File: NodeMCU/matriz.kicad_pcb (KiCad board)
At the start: 2 copper layers, 68 x 68 mm, 26 parts, among them J1 Conn_01x05, J2 Conn_01x02, Q1 Q_NPN_CBE, Q2 Q_NPN_CBE, Q3 Q_NPN_CBE, SW1 SW_Push_Open, SW2 SW_Push, U3 NodeMCU1.0(ESP-12E)

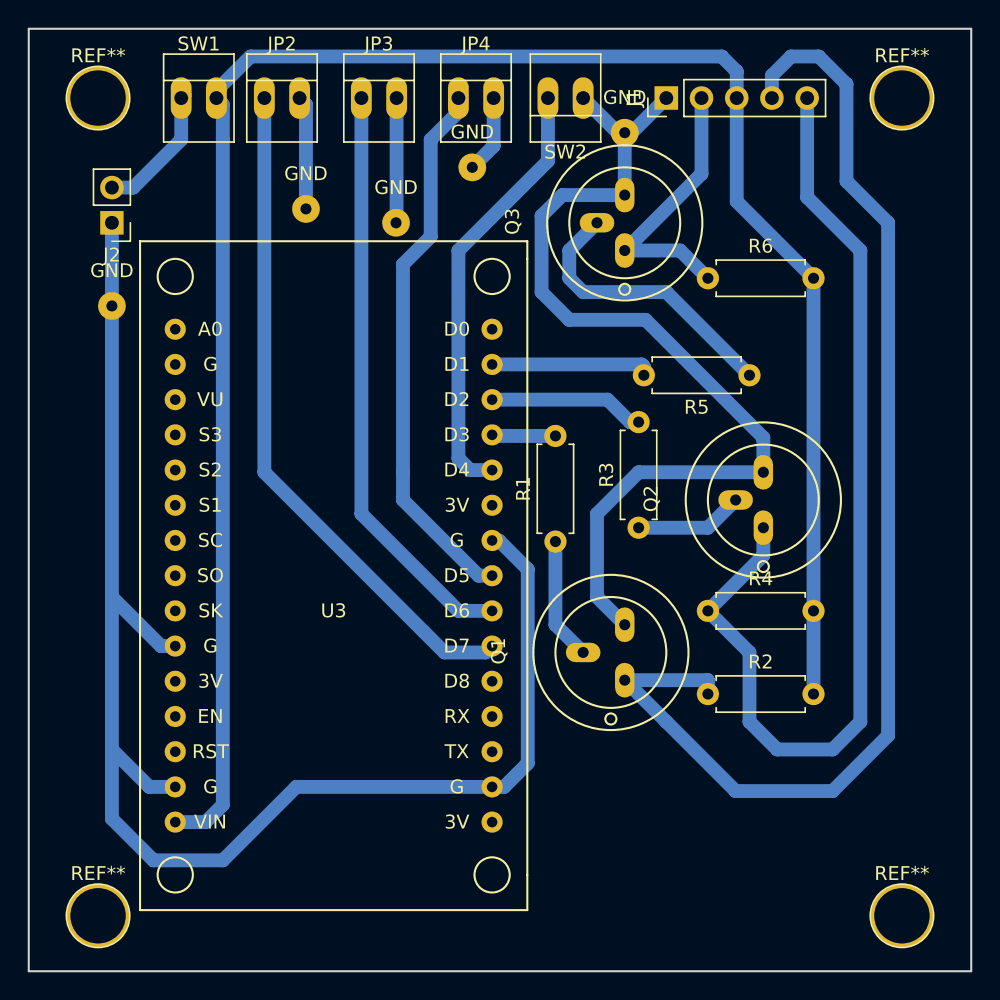
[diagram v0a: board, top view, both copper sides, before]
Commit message: Pads adecuados
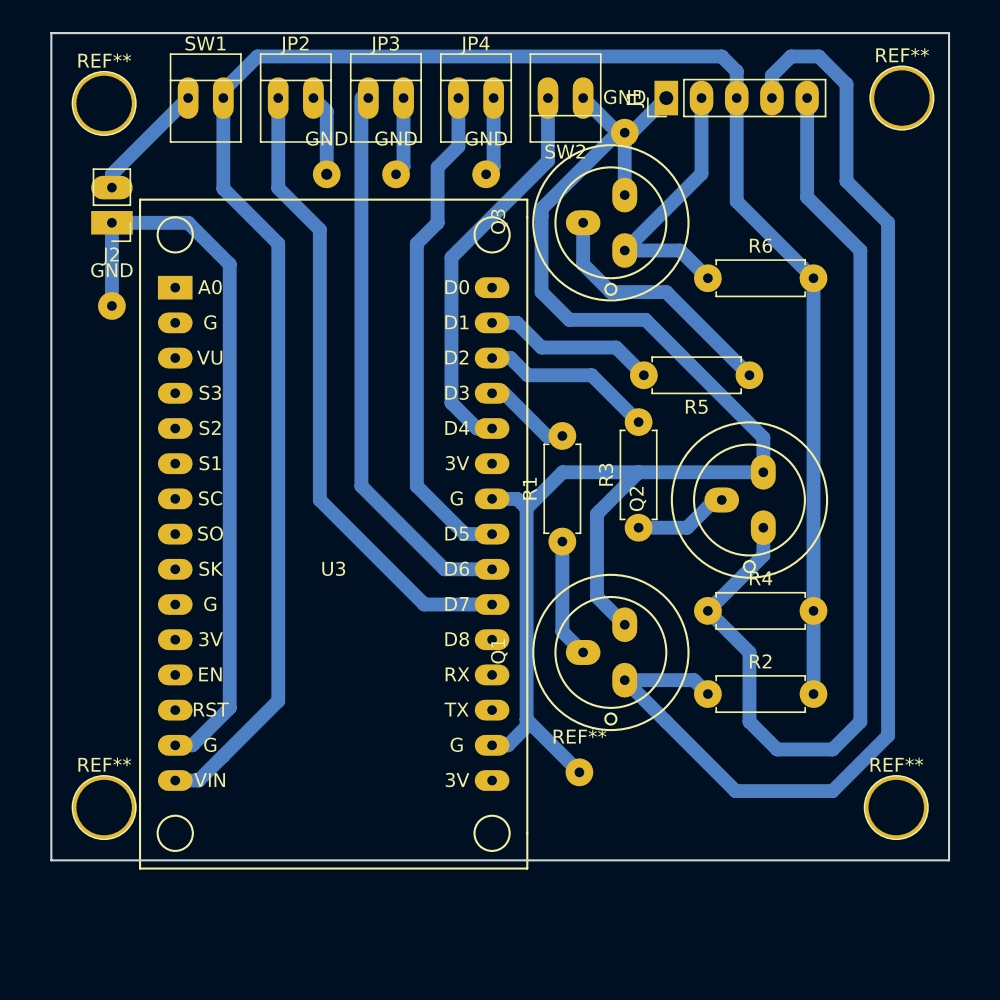
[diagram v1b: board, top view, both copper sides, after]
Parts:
- added REF**: SolderWirePad_single_0-8mmDrill, Wire_Pads:SolderWirePad_single_0-8mmDrill, F.Cu at (125.7, 120.7)
- R1, R3, R5: value 500Ohm -> 10KOhm
- R2, R6: value 1000KOhm -> 10KOhm
- R4: value 1000Ohm -> 10KOhm
- moved REF** 7.82 mm to (91.4, 123.2)
- moved REF** 7.82 mm to (148.6, 123.2)
- moved GND 3.50 mm to (112.5, 77.5)
- moved U3 3.00 mm to (108.0, 106.0)
- moved GND 2.92 mm to (107.5, 77.5)
- moved GND 1.12 mm to (119.0, 77.5)
- moved JP2 1.00 mm to (104.0, 72.0)
- moved Q2 1.00 mm to (138.0, 101.0)
- moved Q3 1.00 mm to (128.0, 81.0)
- moved REF** 0.59 mm to (91.4, 72.4)
- moved JP3 0.50 mm to (110.5, 72.0)
- moved R1 0.50 mm to (124.5, 104.0)
- moved SW1 0.50 mm to (97.5, 72.0)
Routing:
- net /GND: track 199.2 -> 178.4 mm
- net Net-(JP4-Pad1): track 39.3 -> 36.1 mm
- net Net-(JP2-Pad1): track 49.0 -> 45.8 mm
- net Net-(SW2-Pad2): track 31.5 -> 28.6 mm
- net Net-(JP3-Pad1): track 42.3 -> 39.9 mm
- net Net-(Q3-Pad2): track 20.7 -> 18.3 mm
- net Net-(R1-Pad2): track 4.60 -> 6.35 mm
- net Net-(R3-Pad2): track 11.2 -> 12.5 mm
- net /PWR: track 9.92 -> 8.74 mm
- net Net-(Q2-Pad2): track 7.83 -> 6.83 mm
- net Net-(R5-Pad2): track 11.6 -> 12.5 mm
- net /V+: track 141.9 -> 141.2 mm
- net /CLK: track 87.6 -> 87.0 mm
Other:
- board size 68 x 68 mm -> 64.8 x 59.7 mm
